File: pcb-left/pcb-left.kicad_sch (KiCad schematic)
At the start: 92 parts, among them J1 Conn_01x02_Pin, J2 Conn_01x04_Pin, J3 Conn_01x06_MountingPin, SW1 SW_Push, SW2 Rotary_Encoder_Default, U1 XC6206PxxxMR, U2 STM32F401RCTx, Y1 8MHz

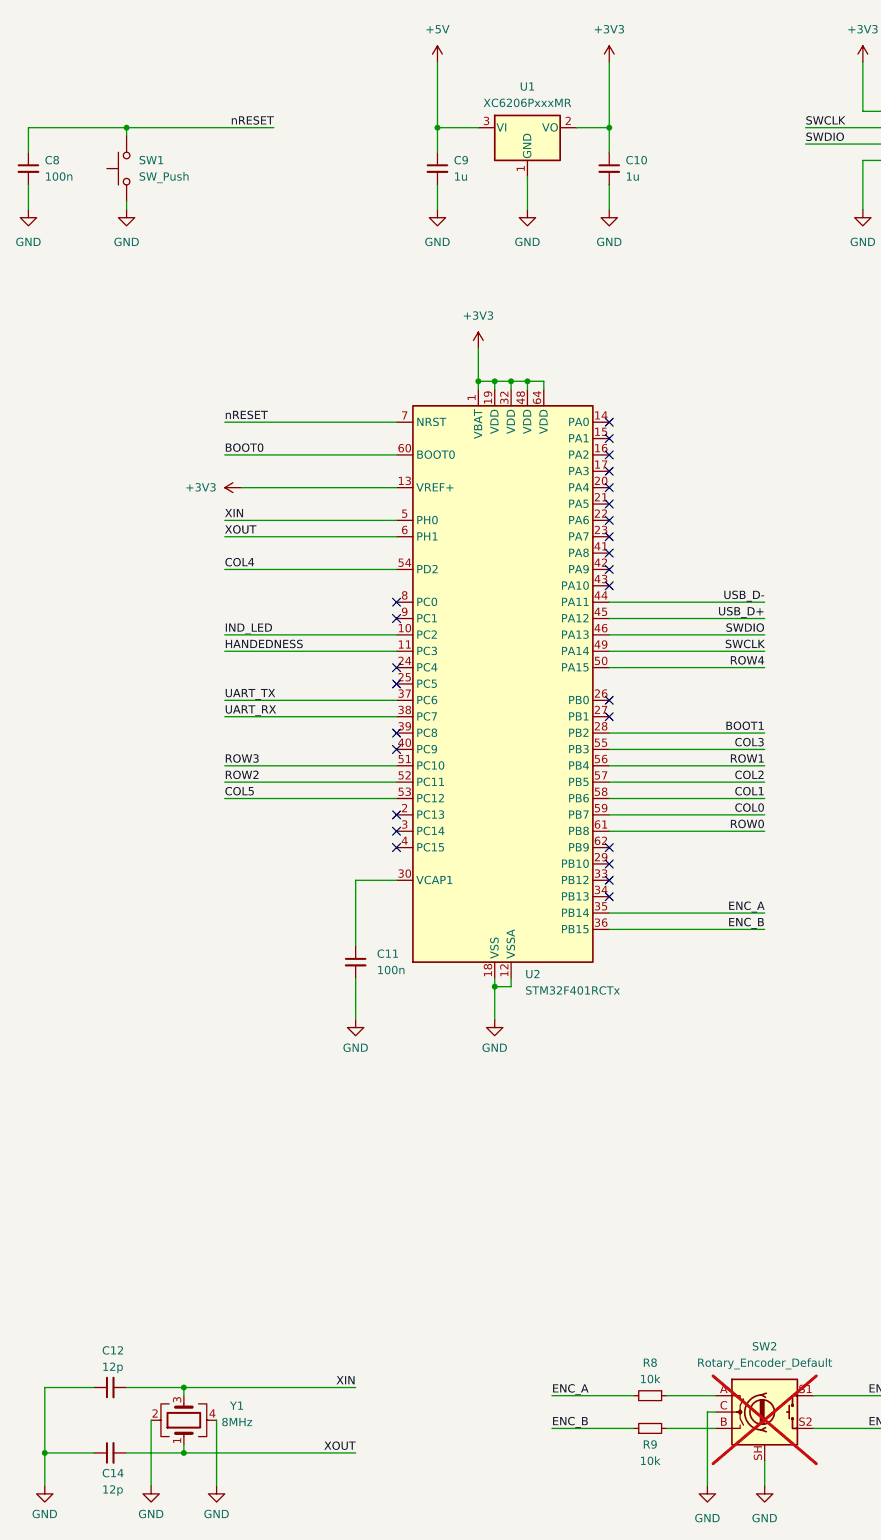
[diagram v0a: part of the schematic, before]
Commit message: intermediate save
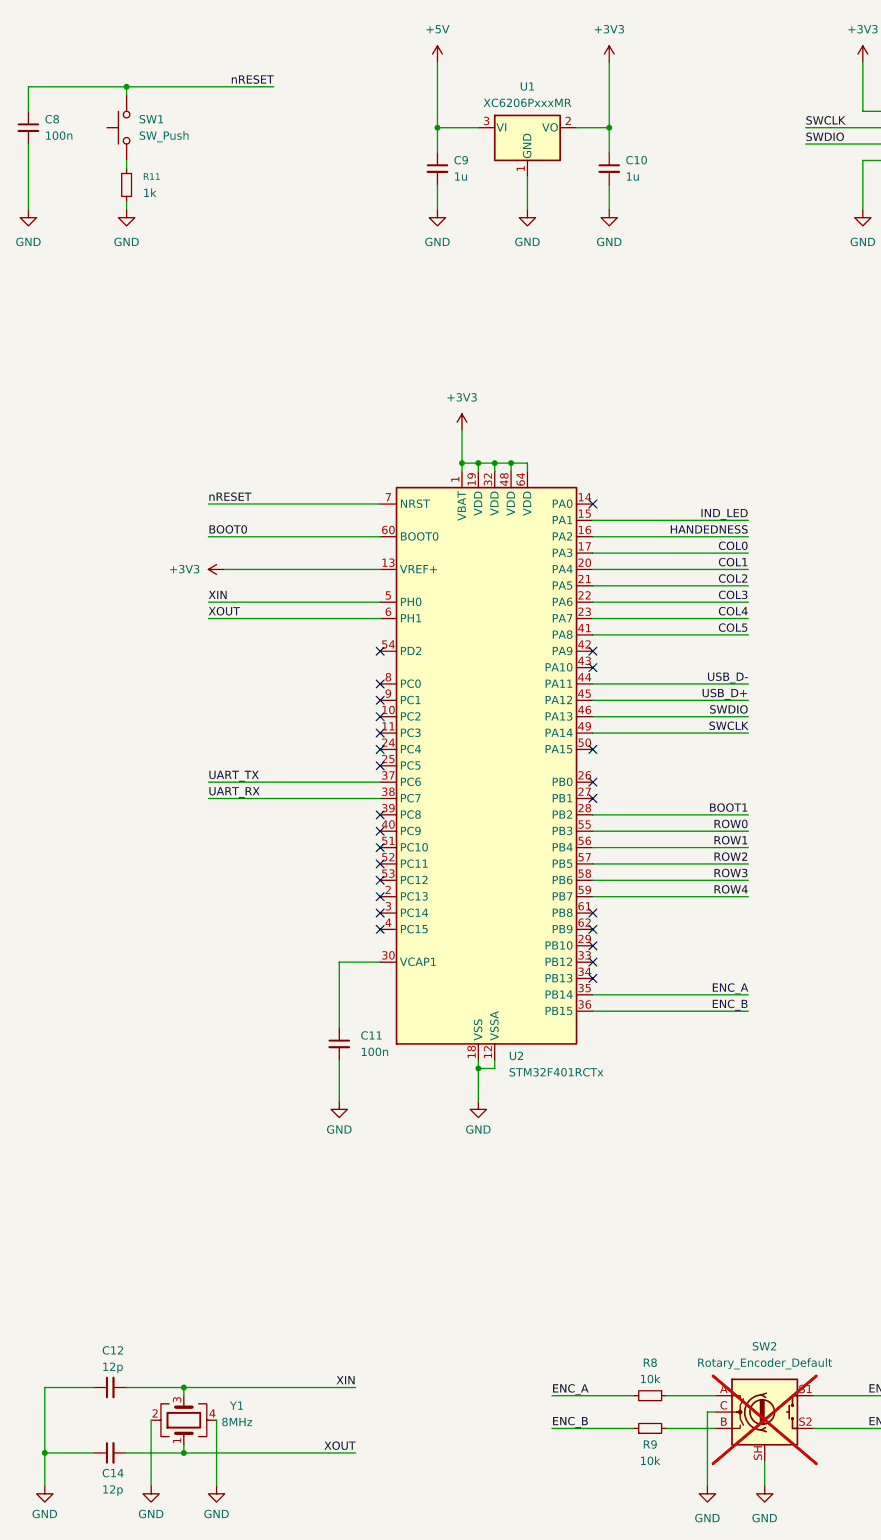
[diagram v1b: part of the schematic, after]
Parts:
- added R11: 1k, Resistor_SMD:R_0603_1608Metric, symbol Device:R_Small
- MX1, MX10, MX11, MX12, MX13, MX14, MX15, MX16, MX17, MX18, MX19, MX2, MX20, MX21, MX22, MX23, MX24, MX25, MX26, MX27, MX28, MX29, MX3, MX4, MX5, MX6, MX7, MX8, MX9: footprint PCM_marbastlib-mx:SW_MX_HS_1u -> PCM_marbastlib-mx:SW_MX_HS_CPG151101S11_1u
- R4, R6: footprint Resistor_SMD:R_0402_1005Metric -> Resistor_SMD:R_0603_1608Metric; now in the parts list
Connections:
- net COL0: now also U2.17 (PA3); no longer U2.59 (PB7)
- net COL1: now also U2.20 (PA4); no longer U2.58 (PB6)
- net COL2: now also U2.21 (PA5); no longer U2.57 (PB5)
- net COL3: now also U2.22 (PA6); no longer U2.55 (PB3)
- net COL4: now also U2.23 (PA7); no longer U2.54 (PD2)
- net COL5: now also U2.41 (PA8); no longer U2.53 (PC12)
- net GND: now also R11.2; no longer SW1.1
- net HANDEDNESS: now also U2.16 (PA2); no longer U2.11 (PC3)
- net IND_LED: now also U2.15 (PA1); no longer U2.10 (PC2)
- net ROW0: now also U2.55 (PB3); no longer U2.61 (PB8)
- net ROW2: now also U2.57 (PB5); no longer U2.52 (PC11)
- net ROW3: now also U2.58 (PB6); no longer U2.51 (PC10)
- net ROW4: now also U2.59 (PB7); no longer U2.50 (PA15)
- new net: R11.1, SW1.1
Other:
- moved on the sheet: C11, C8, SW1, U2
